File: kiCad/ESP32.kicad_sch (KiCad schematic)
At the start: 6 parts, among them J2 TC2030, U2 ESP32-S3-WROOM-1

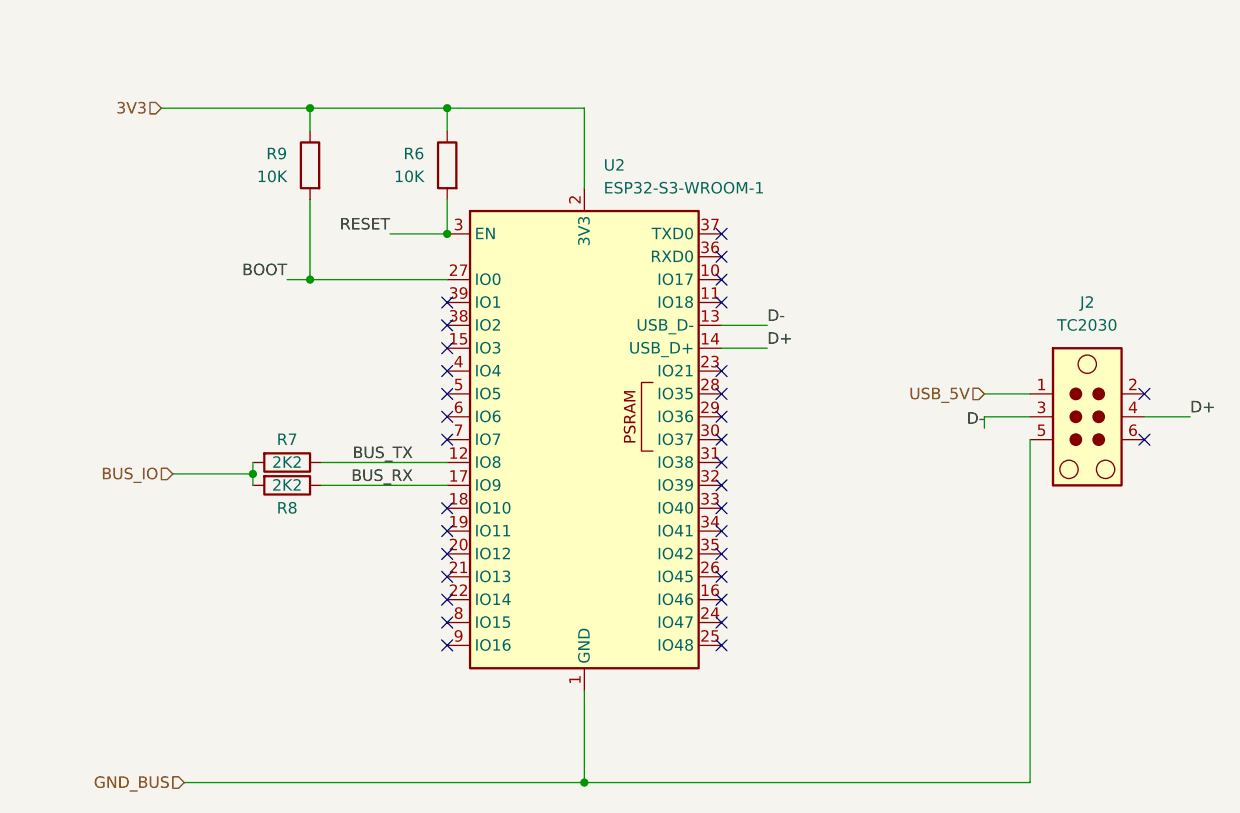
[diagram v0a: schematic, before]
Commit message: Add Pcb
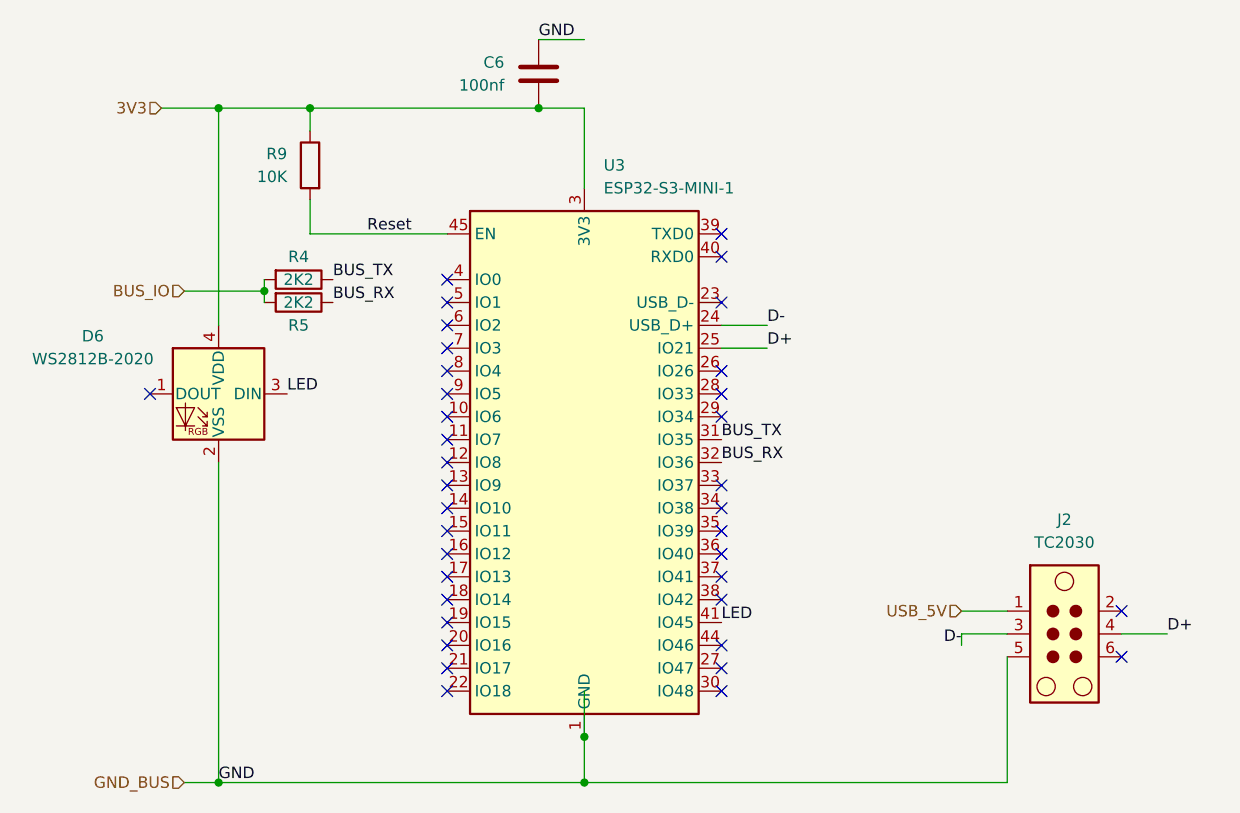
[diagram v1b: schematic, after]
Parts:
- removed R6: 10K, symbol Device:R
- removed R7, R8: 2K2, symbol Device:R
- removed U2: ESP32-S3-WROOM-1, RF_Module:ESP32-S3-WROOM-1, symbol RF_Module:ESP32-S3-WROOM-1
- added C6: 100nf, Capacitor_SMD:C_0603_1608Metric, symbol Device:C
- added D6: WS2812B-2020, 123:LED_SK6805D-OPSCO_2.1x2.1mm, symbol LED:WS2812B-2020
- added R4, R5: 2K2, Resistor_SMD:R_0603_1608Metric, symbol Device:R
- added U3: ESP32-S3-MINI-1, RF_Module:ESP32-S2-MINI-1, symbol RF_Module:ESP32-S3-MINI-1
- R9: footprint (none) -> Resistor_SMD:R_0603_1608Metric; LCSC (none) -> C25744
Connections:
- net 3V3: now also C6.1, D6.4 (VDD), U3.3 (3V3)
- net BUS_IO: now also R4.2, R5.2
- net BUS_RX: now also R5.1, U3.32 (IO36)
- net BUS_TX: now also R4.1, U3.31 (IO35)
- net D+: now also U3.25 (IO21)
- net D-: now also U3.24 (USB_D+)
- net GND_BUS: now also C6.2, D6.2 (VSS), U3.1 (GND), U3.2 (GND), U3.42 (GND), U3.43 (GND), U3.46 (GND), U3.47 (GND), U3.48 (GND), U3.49 (GND), U3.50 (GND), U3.51 (GND), U3.52 (GND), U3.53 (GND), U3.54 (GND), U3.55 (GND), U3.56 (GND), U3.57 (GND), U3.58 (GND), U3.59 (GND), U3.60 (GND), U3.61 (GND), U3.62 (GND), U3.63 (GND), U3.64 (GND), U3.65 (GND)
- net BOOT renamed Reset
- net Reset: now also U3.45 (EN)
- new net LED: D6.3 (DIN), U3.41 (IO45)
- no-connect marks 33 -> 37
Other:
- moved on the sheet: J2
